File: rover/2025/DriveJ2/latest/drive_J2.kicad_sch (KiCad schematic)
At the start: 54 parts, among them J1 USB_C_USB4105-GF-A, J10 Jumper PWR, J2 XT30PW-F, J3 Eth-Horiz, J4 Eth-Horiz, J5 Conn_01x03, J6 Conn_01x02, J8 Conn_01x03, J9 Conn_01x06, SW1 TS09-63-25-WT-160-SMT-TR, SW2 TS09-63-25-WT-160-SMT-TR, SW3 TS09-63-25-WT-160-SMT-TR, SW4 TS09-63-25-WT-160-SMT-TR, U1 TVS-SMDB03CE3, U2 ESP32-S3-WROVER, U3 XT60PM-F, U4 XT60PW-M, U5 LDO-TLV74033PDBVR, U6 SN65HVD232, U7 SN65HVD232, U8 LDO-LM7805MPX/NOPB

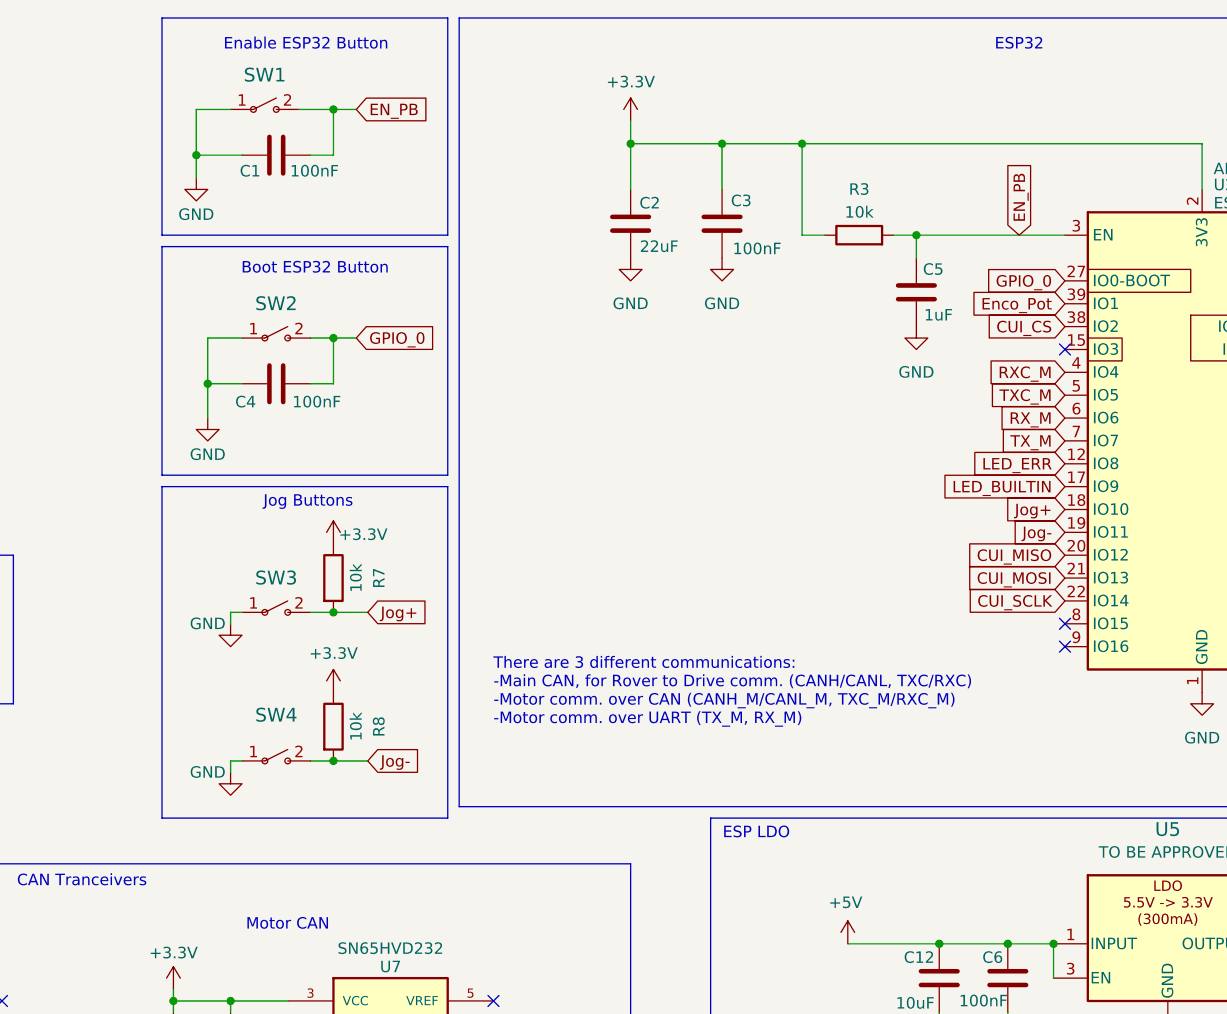
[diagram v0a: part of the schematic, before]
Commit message: Upgraded version of DriveJ2
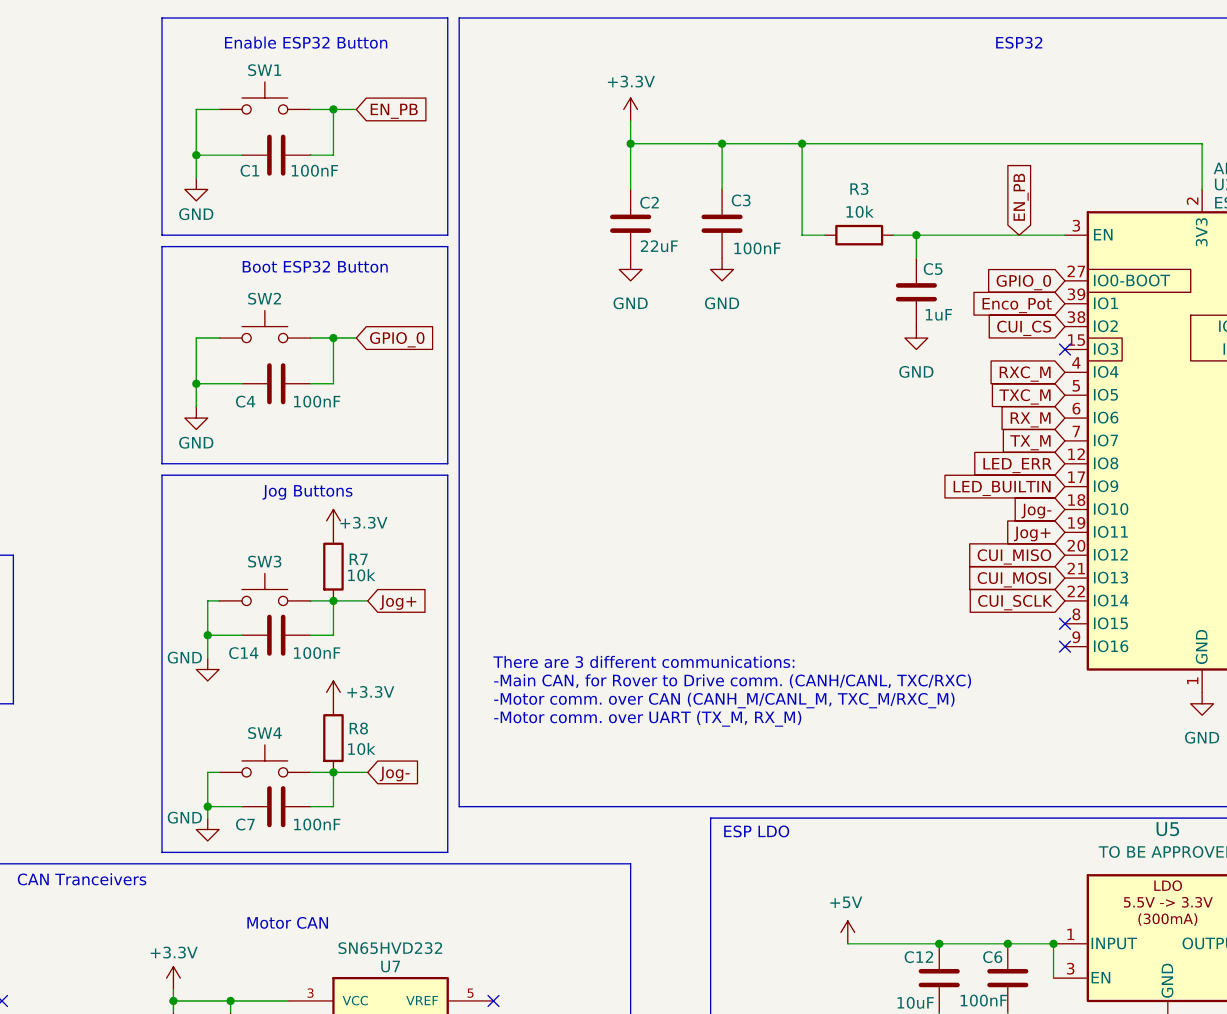
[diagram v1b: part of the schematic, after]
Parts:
- removed SW1, SW2, SW3, SW4: TS09-63-25-WT-160-SMT-TR, Button_Switch_SMD:SW_DIP_SPSTx01_Slide_6.7x4.1mm_W8.61mm_P2.54mm_LowProfile, symbol Rover_LIB:PushButton-TS09-63-25-WT-160-SMT-TR
- added C14, C7: 100nF, Capacitor_SMD:C_0805_2012Metric_Pad1.18x1.45mm_HandSolder, symbol Rover_LIB:C_0805
- added SW1, SW2, SW3, SW4: SW-PTS815SJM250SMTRLFS, RoverFootprint:SW-PTS815 SJM250SMTRLFS, symbol Rover_LIB:SW-PTS815SJM250SMTRLFS
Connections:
- net EN_PB: now also SW1.4
- net GND: now also C14.1, C7.1, SW1.1, SW1.2, SW2.1, SW2.2, SW3.1, SW3.2, SW4.1, SW4.2
- net GPIO_0: now also SW2.4
- net Jog+: now also U2.19 (IO11), C14.2, SW3.4; no longer U2.18 (IO10)
- net Jog-: now also U2.18 (IO10), C7.2, SW4.4; no longer U2.19 (IO11)
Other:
- moved on the sheet: R7, R8
